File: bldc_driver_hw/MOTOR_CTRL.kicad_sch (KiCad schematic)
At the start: 11 parts

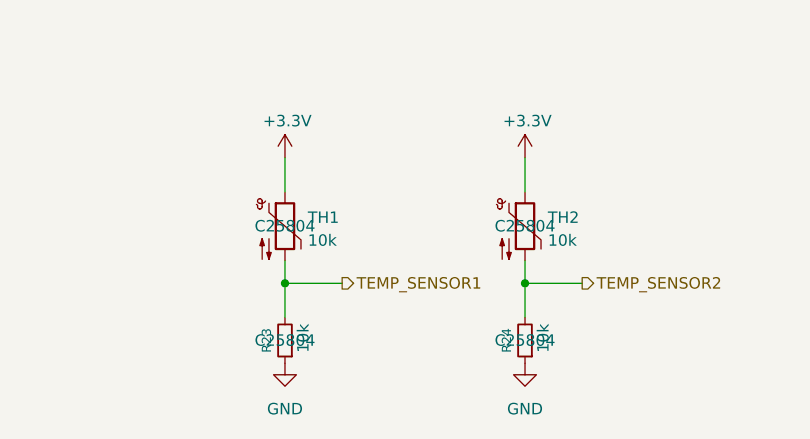
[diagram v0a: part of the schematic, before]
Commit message: finished
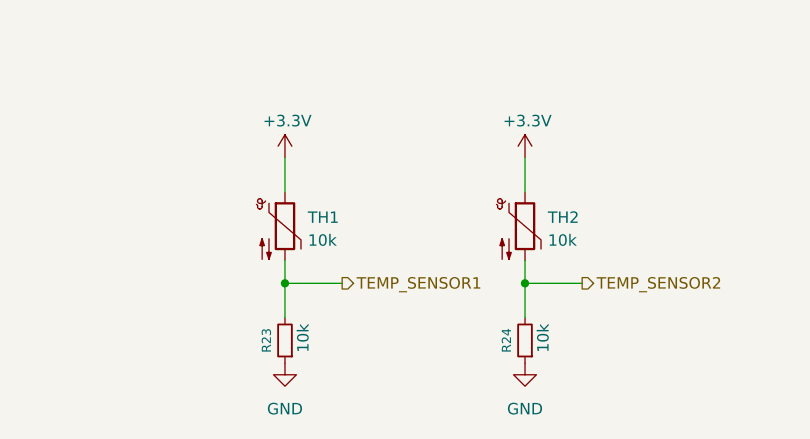
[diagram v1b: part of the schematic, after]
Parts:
- C39, C40, C41, C45, TP23, TP24, TP25: now left out of the parts list
- TH1, TH2: LCSC C25804 -> (none); now left out of the parts list
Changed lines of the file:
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@@
 		(unit 1)
 		(exclude_from_sim no)
-		(in_bom yes)
+		(in_bom no)
 		(on_board yes)
 		(dnp no)
@@
 		(unit 1)
 		(exclude_from_sim no)
-		(in_bom yes)
+		(in_bom no)
 		(on_board yes)
 		(dnp no)
@@
 		(unit 1)
 		(exclude_from_sim no)
-		(in_bom yes)
+		(in_bom no)
 		(on_board yes)
 		(dnp no)
@@
 			)
 		)
-		(property "LCSC" "C25804"
+		(property "LCSC" ""
 			(at 109.22 172.72 0)
 			(effects
@@
 		(unit 1)
 		(exclude_from_sim no)
-		(in_bom yes)
+		(in_bom no)
 		(on_board yes)
 		(dnp no)
@@
 			)
 		)
-		(property "LCSC" "C25804"
+		(property "LCSC" ""
 			(at 135.89 172.72 0)
 			(effects
@@
 		)
 		(property "LCSC" "C25804"
-			(at 135.89 185.42 0)
-			(effects
-				(font
-					(size 1.27 1.27)
-				)
+			(at 132.08 186.436 0)
+			(effects
+				(font
+					(size 1.27 1.27)
+				)
+				(hide yes)
 			)
 		)
@@
 		(unit 1)
 		(exclude_from_sim no)
-		(in_bom yes)
+		(in_bom no)
 		(on_board yes)
 		(dnp no)
@@
 		)
 		(property "LCSC" "C25804"
-			(at 109.22 185.42 0)
-			(effects
-				(font
-					(size 1.27 1.27)
-				)
+			(at 104.902 185.928 90)
+			(effects
+				(font
+					(size 1.27 1.27)
+				)
+				(hide yes)
 			)
 		)
@@
 		(unit 1)
 		(exclude_from_sim no)
-		(in_bom yes)
+		(in_bom no)
 		(on_board yes)
 		(dnp no)
@@
 		(unit 1)
 		(exclude_from_sim no)
-		(in_bom yes)
+		(in_bom no)
 		(on_board yes)
 		(dnp no)
@@
 		(unit 1)
 		(exclude_from_sim no)
-		(in_bom yes)
+		(in_bom no)
 		(on_board yes)
 		(dnp no)
@@
 		(unit 1)
 		(exclude_from_sim no)
-		(in_bom yes)
-		(on_board yes)
-		(dnp no)
+		(in_bom no)
+		(on_board yes)
+		(dnp no)
